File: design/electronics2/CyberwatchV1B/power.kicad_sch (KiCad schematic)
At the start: 6 parts, among them J3 Conn_01x02_Socket, Q1 AO3401A, SW6 SW_power, U4 MAX17048

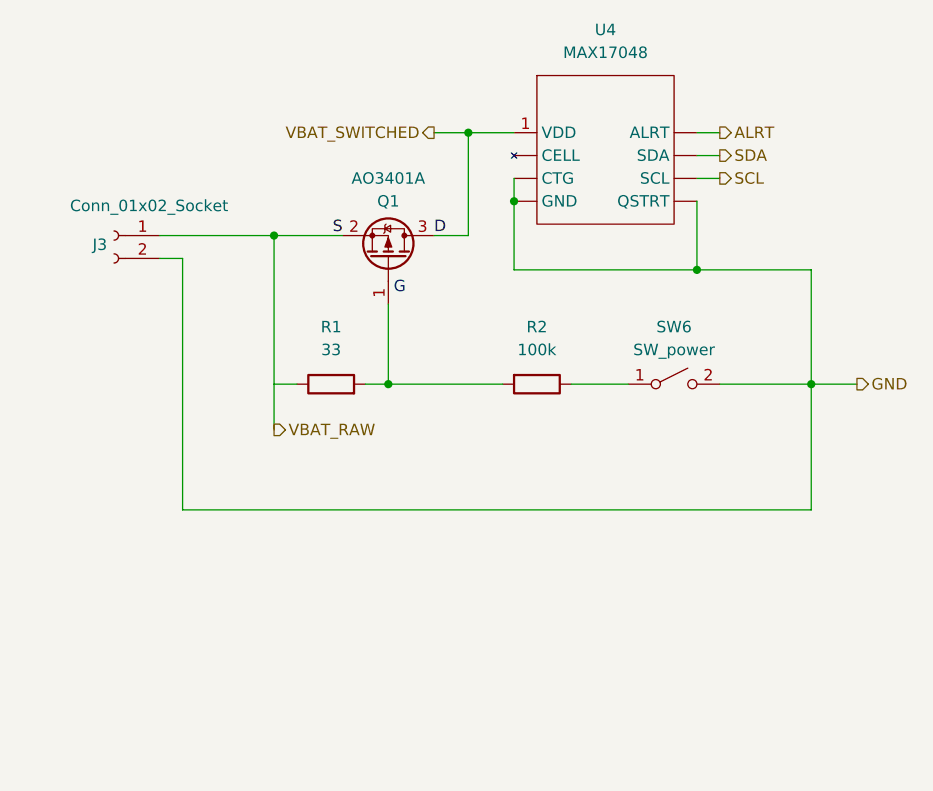
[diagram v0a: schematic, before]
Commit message: power schematic finalisation
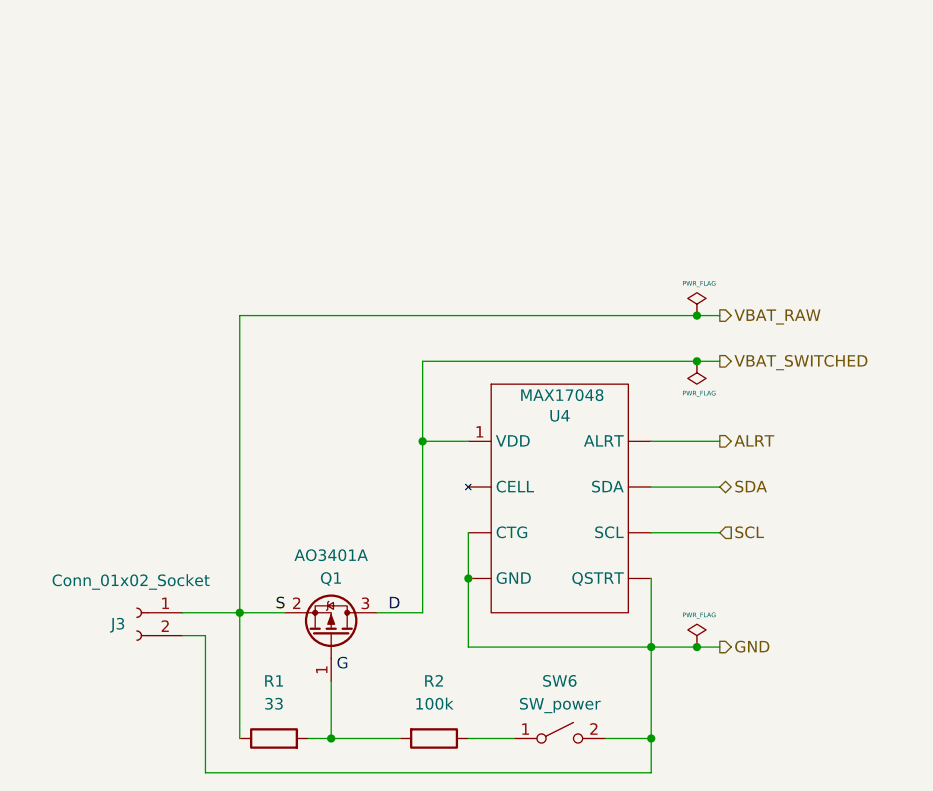
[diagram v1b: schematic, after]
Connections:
- net VBAT_RAW: now also R1.1
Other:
- moved on the sheet: J3, Q1, R1, R2, SW6, U4
